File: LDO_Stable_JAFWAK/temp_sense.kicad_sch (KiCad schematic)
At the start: 6 parts, among them U2 TMP235A2DBZR

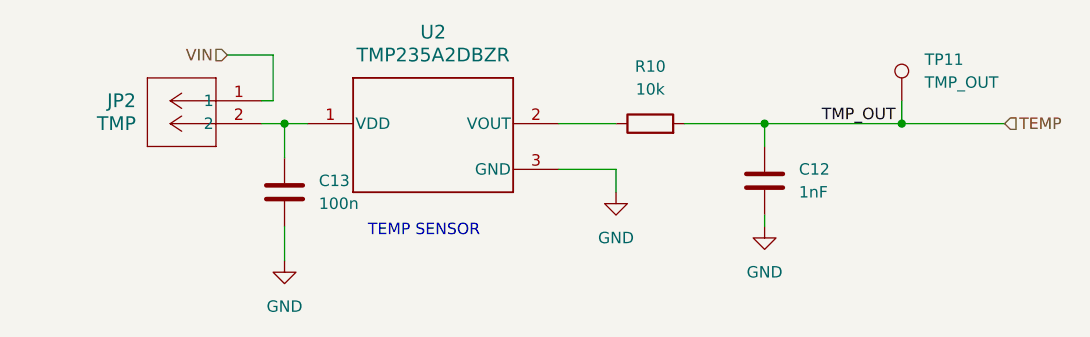
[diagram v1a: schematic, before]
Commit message: Started Layout
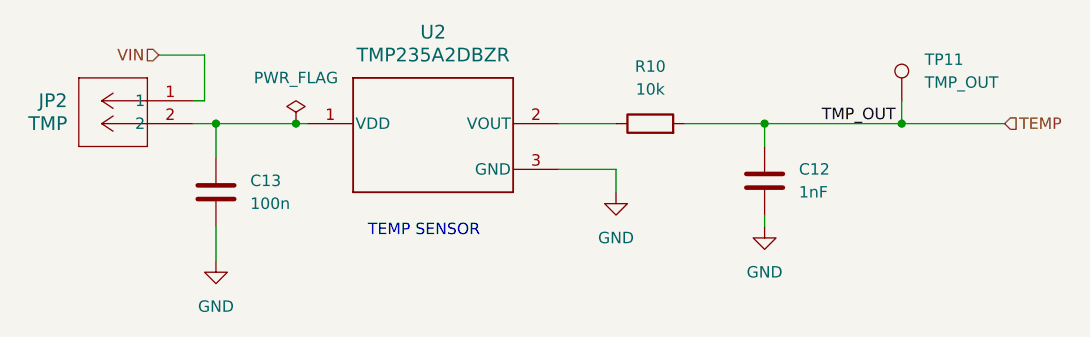
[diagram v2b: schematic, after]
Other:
- moved on the sheet: C13, JP2
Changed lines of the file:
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@@
 	)
 	(junction
-		(at 110.49 77.47)
+		(at 102.87 77.47)
 		(diameter 0)
 		(color 0 0 0 0)
@@
 		(color 0 0 0 0)
 	)
+	(junction
+		(at 111.76 77.47)
+		(diameter 0)
+		(color 0 0 0 0)
+	)
 	(wire
 		(pts
@@
 	(wire
 		(pts
-			(xy 104.14 69.85) (xy 109.22 69.85)
+			(xy 96.52 69.85) (xy 101.6 69.85)
 		)
 		(stroke
@@
 	(wire
 		(pts
-			(xy 109.22 74.93) (xy 107.95 74.93)
-		)
-		(stroke
-			(width 0)
-			(type default)
-		)
-	)
-	(wire
-		(pts
-			(xy 109.22 69.85) (xy 109.22 74.93)
-		)
-		(stroke
-			(width 0)
-			(type default)
-		)
-	)
-	(wire
-		(pts
-			(xy 110.49 88.9) (xy 110.49 92.71)
-		)
-		(stroke
-			(width 0)
-			(type default)
-		)
-	)
-	(wire
-		(pts
-			(xy 110.49 77.47) (xy 113.03 77.47)
+			(xy 101.6 74.93) (xy 100.33 74.93)
+		)
+		(stroke
+			(width 0)
+			(type default)
+		)
+	)
+	(wire
+		(pts
+			(xy 101.6 69.85) (xy 101.6 74.93)
+		)
+		(stroke
+			(width 0)
+			(type default)
+		)
+	)
+	(wire
+		(pts
+			(xy 102.87 88.9) (xy 102.87 92.71)
+		)
+		(stroke
+			(width 0)
+			(type default)
+		)
+	)
+	(wire
+		(pts
+			(xy 102.87 77.47) (xy 111.76 77.47)
 		)
 		(stroke
@@
 	(wire
 		(pts
-			(xy 110.49 77.47) (xy 110.49 81.28)
-		)
-		(stroke
-			(width 0)
-			(type default)
-		)
-	)
-	(wire
-		(pts
-			(xy 107.95 77.47) (xy 110.49 77.47)
+			(xy 102.87 77.47) (xy 102.87 81.28)
+		)
+		(stroke
+			(width 0)
+			(type default)
+		)
+	)
+	(wire
+		(pts
+			(xy 100.33 77.47) (xy 102.87 77.47)
 		)
 		(stroke
@@
 		(pts
 			(xy 163.83 77.47) (xy 163.83 80.01)
+		)
+		(stroke
+			(width 0)
+			(type default)
+		)
+	)
+	(wire
+		(pts
+			(xy 111.76 77.47) (xy 113.03 77.47)
 		)
 		(stroke
@@
 	(hierarchical_label "VIN"
 		(shape input)
-		(at 104.14 69.85 180)
+		(at 96.52 69.85 180)
 		(effects
 			(font
@@
 	(symbol
 		(lib_id "power:GND")
-		(at 110.49 92.71 0)
+		(at 102.87 92.71 0)
 		(unit 1)
 		(body_style 1)
@@
 		(fields_autoplaced yes)
 		(property "Reference" "#PWR019"
-			(at 110.49 99.06 0)
+			(at 102.87 99.06 0)
 			(hide yes)
 			(show_name no)
@@
 		)
 		(property "Value" "GND"
-			(at 110.49 97.79 0)
+			(at 102.87 97.79 0)
 			(show_name no)
 			(do_not_autoplace no)
@@
 		)
 		(property "Footprint" ""
-			(at 110.49 92.71 0)
+			(at 102.87 92.71 0)
 			(hide yes)
 			(show_name no)
@@
 		)
 		(property "Datasheet" ""
-			(at 110.49 92.71 0)
+			(at 102.87 92.71 0)
 			(hide yes)
 			(show_name no)
@@
 		)
 		(property "Description" "Power symbol creates a global label with name \"GND\" , ground"
-			(at 110.49 92.71 0)
+			(at 102.87 92.71 0)
 			(hide yes)
 			(show_name no)
@@
 	(symbol
 		(lib_id "Device:C")
-		(at 110.49 85.09 0)
+		(at 102.87 85.09 0)
 		(unit 1)
 		(body_style 1)
@@
 		(fields_autoplaced yes)
 		(property "Reference" "C13"
-			(at 114.3 83.8199 0)
+			(at 106.68 83.8199 0)
 			(show_name no)
 			(do_not_autoplace no)
@@
 		)
 		(property "Value" "100n"
-			(at 114.3 86.3599 0)
+			(at 106.68 86.3599 0)
 			(show_name no)
 			(do_not_autoplace no)
@@
 		)
 		(property "Footprint" "Capacitor_SMD:C_0805_2012Metric_Pad1.18x1.45mm_HandSolder"
-			(at 111.4552 88.9 0)
+			(at 103.8352 88.9 0)
 			(hide yes)
 			(show_name no)
@@
 		)
 		(property "Datasheet" "https://yageogroup.com/content/datasheet/asset/file/KEM_C1002_X7R_SMD"
-			(at 110.49 85.09 0)
+			(at 102.87 85.09 0)
 			(hide yes)
 			(show_name no)
@@
 		)
 		(property "Description" "CAP CER 1000PF 50V X7R 0805"
-			(at 110.49 85.09 0)
+			(at 102.87 85.09 0)
 			(hide yes)
 			(show_name no)
@@
 		)
 		(property "Manufacturer" "KEMET"
-			(at 110.49 85.09 0)
+			(at 102.87 85.09 0)
 			(hide yes)
 			(show_name no)
@@
 		)
 		(property "Manufacturer Part Number" "C0805C102K5RACTU"
-			(at 110.49 85.09 0)
+			(at 102.87 85.09 0)
 			(hide yes)
 			(show_name no)
@@
 		)
 		(property "Distributer Link 1" "https://www.digikey.com/en/products/detail/kemet/C0805C102K5RACTU/411146"
-			(at 110.49 85.09 0)
+			(at 102.87 85.09 0)
 			(hide yes)
 			(show_name no)
@@
 		)
 		(property "Distributer Link 2" "https://www.mouser.com/en/ProductDetail/KEMET/C0805C102K5RACTU?qs=nyGfpDADWE7v2OrzBT8v1g%3D%3D"
-			(at 110.49 85.09 0)
+			(at 102.87 85.09 0)
 			(hide yes)
 			(show_name no)
@@
 	(symbol
 		(lib_id "PEC02SAAN:PEC02SAAN")
-		(at 107.95 74.93 0)
+		(at 100.33 74.93 0)
 		(mirror y)
 		(unit 1)
@@
 		(dnp no)
 		(property "Reference" "JP2"
-			(at 93.98 74.9299 0)
+			(at 86.36 74.9299 0)
 			(show_name no)
 			(do_not_autoplace no)
@@
 		)
 		(property "Value" "TMP"
-			(at 93.98 77.4699 0)
+			(at 86.36 77.4699 0)
 			(show_name no)
 			(do_not_autoplace no)
@@
 		)
 		(property "Footprint" "Connector_PinHeader_2.54mm:PinHeader_1x02_P2.54mm_Vertical"
-			(at 107.95 74.93 0)
+			(at 100.33 74.93 0)
 			(hide yes)
 			(show_name no)
@@
 		)
 		(property "Datasheet" "PEC02SAAN"
-			(at 107.95 74.93 0)
+			(at 100.33 74.93 0)
 			(hide yes)
 			(show_name no)
@@
 		)
 		(property "Description" "CONN HEADER VERT 2POS 2.54MM"
-			(at 107.95 74.93 0)
+			(at 100.33 74.93 0)
 			(hide yes)
 			(show_name no)
@@
 		)
 		(property "Manufacturer" "Sullins Connector Solutions"
-			(at 107.95 74.93 0)
+			(at 100.33 74.93 0)
 			(hide yes)
 			(show_name no)
@@
 		)
 		(property "Manufacturer Part Number" "PEC02SAAN"
-			(at 107.95 74.93 0)
+			(at 100.33 74.93 0)
 			(hide yes)
 			(show_name no)
@@
 		)
 		(property "Distributer Link 1" "https://www.digikey.com/en/products/detail/sullins-connector-solutions/PEC02SAAN/859155?s=N4IgTCBcDaIAoFEDCAGMBlAgpgciAugL5A"
-			(at 107.95 74.93 0)
+			(at 100.33 74.93 0)
 			(hide yes)
 			(show_name no)
@@
 		)
 		(property "Distributer Link 2" ""
-			(at 107.95 74.93 0)
+			(at 100.33 74.93 0)
 			(hide yes)
 			(show_name no)
@@
 					(unit 1)
 				)
+			)
+		)
+	)
+	(symbol
+		(lib_id "power:PWR_FLAG")
+		(at 111.76 77.47 0)
+		(unit 1)
+		(body_style 1)
+		(exclude_from_sim no)
+		(in_bom yes)
+		(on_board yes)
+		(in_pos_files yes)
+		(dnp no)
+		(fields_autoplaced yes)
+		(property "Reference" "#FLG07"
+			(at 111.76 75.565 0)
+			(hide yes)
+			(show_name no)
+			(do_not_autoplace no)
+			(effects
+				(font
+					(size 1.27 1.27)
+				)
+			)
+		)
+		(property "Value" "PWR_FLAG"
+			(at 111.76 72.39 0)
+			(show_name no)
+			(do_not_autoplace no)
+			(effects
+				(font
+					(size 1.27 1.27)
+				)
+			)
+		)
+		(property "Footprint" ""
+			(at 111.76 77.47 0)
+			(hide yes)
+			(show_name no)
+			(do_not_autoplace no)
+			(effects
+				(font
+					(size 1.27 1.27)
+				)
+			)
+		)
+		(property "Datasheet" ""
+			(at 111.76 77.47 0)
+			(hide yes)
+			(show_name no)
+			(do_not_autoplace no)
+			(effects
+				(font
+					(size 1.27 1.27)
+				)
+			)
+		)
+		(property "Description" "Special symbol for telling ERC where power comes from"
+			(at 111.76 77.47 0)
+			(hide yes)
+			(show_name no)
+			(do_not_autoplace no)
+			(effects
+				(font
+					(size 1.27 1.27)
+				)
+			)
+		)
+		(pin "1"
+		)
+		(instances
+			(project "LDO_Stable_JAFWAK"
+				(path "/e797984e-8841-4b55-a934-93c9429b6b10/ff44080c-9e84-4b6d-8105-be8b15417474"
+					(reference "#FLG07")
+					(unit 1)
+				)
